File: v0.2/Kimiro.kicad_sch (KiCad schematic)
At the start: 24 parts, among them J1 Conn_01x04, J2 USB_C_Left, J3 Left, J4 Right, Q1 AO3407, U1 TP4054, U3 MS88FS3, U4 XC6220B331MR

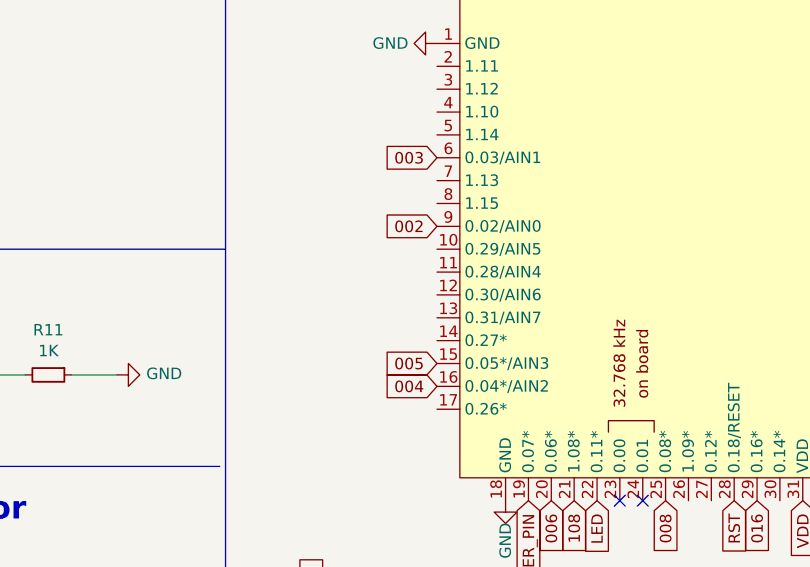
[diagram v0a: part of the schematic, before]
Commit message: Cập nhật file PCB
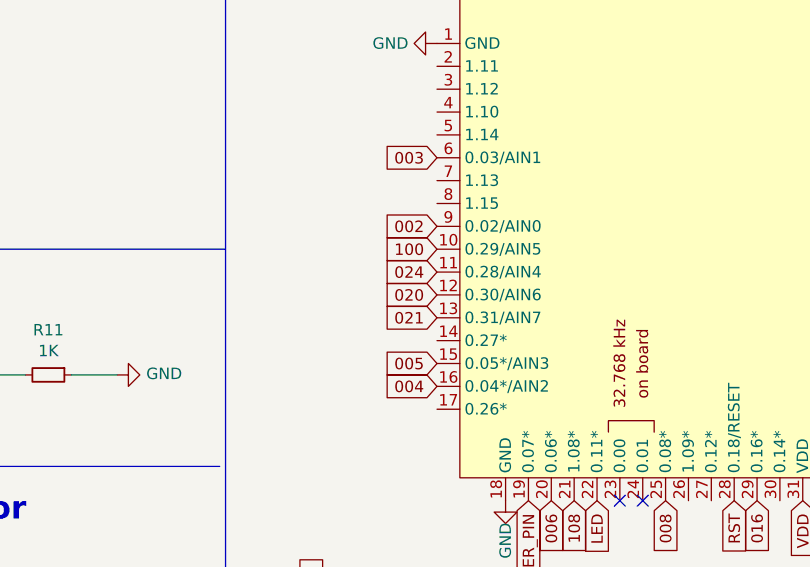
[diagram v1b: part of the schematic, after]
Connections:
- net 020: now also U3.12 (0.30/AIN6)
- net 021: now also U3.13 (0.31/AIN7)
- net 024: now also U3.11 (0.28/AIN4)
- net 100: now also U3.10 (0.29/AIN5)
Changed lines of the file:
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@@
+    )
+  )
+  (global_label "020" (shape input) (at 92.71 133.35 180) (fields_autoplaced)
+    (effects (font (size 1.27 1.27)) (justify right))
+    (property "Intersheet References" "${INTERSHEET_REFS}" (id 0) (at 86.6683 133.4294 0)
+      (effects (font (size 1.27 1.27)) (justify right) hide)
     )
   )
@@
     )
   )
+  (global_label "100" (shape input) (at 92.71 128.27 180) (fields_autoplaced)
+    (effects (font (size 1.27 1.27)) (justify right))
+    (property "Intersheet References" "${INTERSHEET_REFS}" (id 0) (at 86.6683 128.1906 0)
+      (effects (font (size 1.27 1.27)) (justify right) hide)
+    )
+  )
   (global_label "VDD" (shape input) (at 91.44 170.18 90) (fields_autoplaced)
     (effects (font (size 1.27 1.27)) (justify left))
@@
     )
   )
+  (global_label "024" (shape input) (at 92.71 130.81 180) (fields_autoplaced)
+    (effects (font (size 1.27 1.27)) (justify right))
+    (property "Intersheet References" "${INTERSHEET_REFS}" (id 0) (at 86.6683 130.8894 0)
+      (effects (font (size 1.27 1.27)) (justify right) hide)
+    )
+  )
   (global_label "DCCH" (shape input) (at 138.43 156.21 270) (fields_autoplaced)
     (effects (font (size 1.27 1.27)) (justify right))
@@
       (effects (font (size 1.27 1.27)) (justify right) hide)
     )
+  )
+  (global_label "021" (shape input) (at 92.71 135.89 180) (fields_autoplaced)
+    (effects (font (size 1.27 1.27)) (justify right))
+    (property "Intersheet References" "${INTERSHEET_REFS}" (id 0) (at 86.6683 135.8106 0)
+      (effects (font (size 1.27 1.27)) (justify right) hide)
+    )
